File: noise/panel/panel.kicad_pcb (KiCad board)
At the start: 2 copper layers, 33 x 99.1 mm, 4 parts

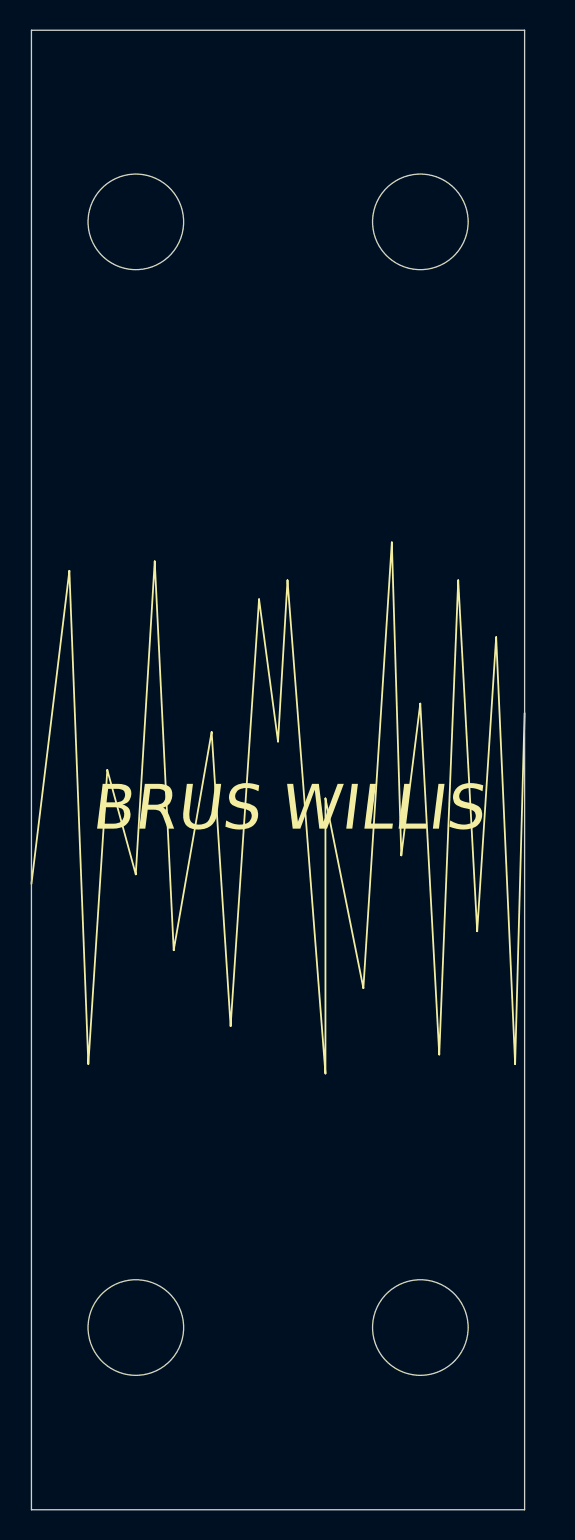
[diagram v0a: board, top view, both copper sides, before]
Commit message: Changes
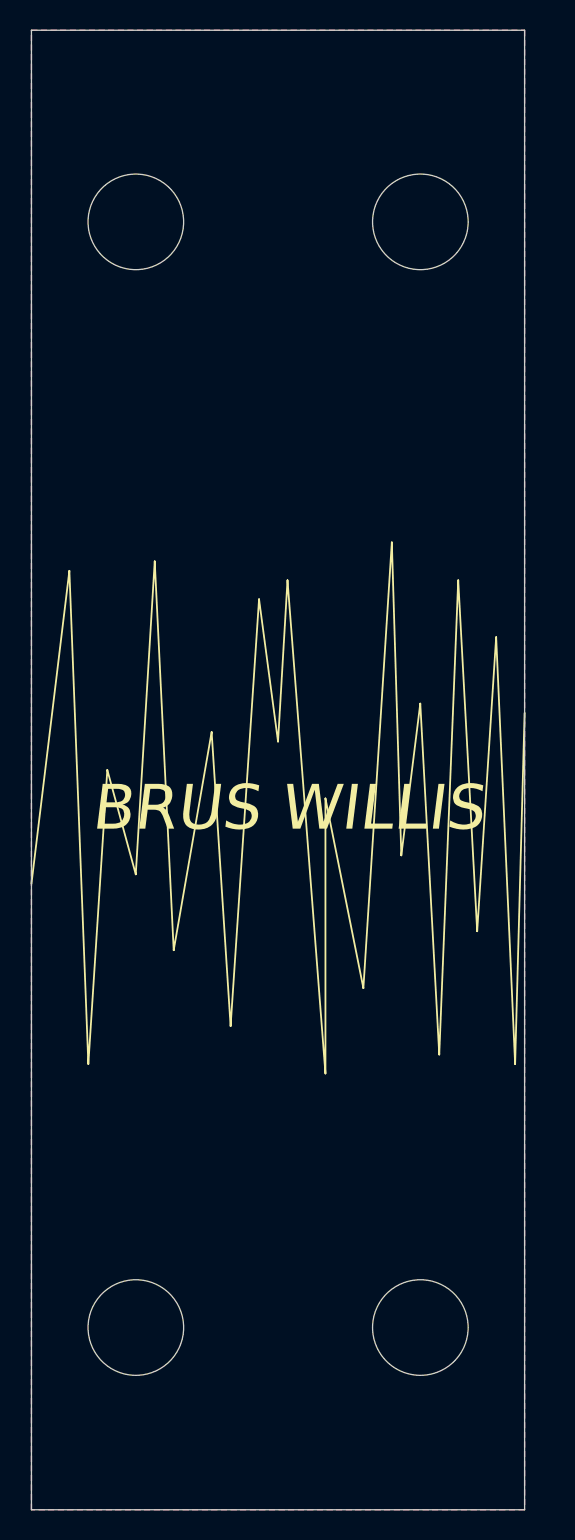
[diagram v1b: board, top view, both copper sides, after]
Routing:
- added copper zone on B.Cu, net (none)
- added copper zone on F.Cu, net (none)
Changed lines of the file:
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@@
   (general
     (thickness 1.6)
-    (drawings 29)
+    (drawings 28)
     (tracks 0)
     (zones 0)
@@
     (pcbplotparams
       (layerselection 0x010fc_ffffffff)
-      (usegerberextensions false)
-      (usegerberattributes true)
-      (usegerberadvancedattributes true)
-      (creategerberjobfile true)
+      (usegerberextensions true)
+      (usegerberattributes false)
+      (usegerberadvancedattributes false)
+      (creategerberjobfile false)
       (excludeedgelayer true)
       (linewidth 0.100000)
@@
       (plotinvisibletext false)
       (padsonsilk false)
-      (subtractmaskfromsilk false)
+      (subtractmaskfromsilk true)
       (outputformat 1)
       (mirror false)
-      (drillshape 1)
+      (drillshape 0)
       (scaleselection 1)
-      (outputdirectory ""))
+      (outputdirectory "plot"))
   )
   (net 0 "")
@@
       (effects (font (size 1 1) (thickness 0.15)))
     )
-    (fp_text user %R (at 0.3 0) (layer F.Fab) hide
-      (effects (font (size 1 1) (thickness 0.15)))
-    )
-    (fp_circle (center 0 0) (end 6.4 0) (layer Cmts.User) (width 0.15))
-    (fp_circle (center 0 0) (end 6.65 0) (layer F.CrtYd) (width 0.05))
+    (fp_circle (center 0 0) (end 6.4 0) (layer Cmts.User) (width 0.15))
+    (fp_circle (center 0 0) (end 6.65 0) (layer F.CrtYd) (width 0.05))
+    (fp_text user %R (at 0.3 0) (layer F.Fab) hide
+      (effects (font (size 1 1) (thickness 0.15)))
+    )
     (pad 1 np_thru_hole circle (at 0 0) (size 6.4 6.4) (drill 6.4) (layers *.Cu *.Mask))
   )
@@
       (effects (font (size 1 1) (thickness 0.15)))
     )
-    (fp_text user %R (at 0.3 0) (layer F.Fab) hide
-      (effects (font (size 1 1) (thickness 0.15)))
-    )
-    (fp_circle (center 0 0) (end 6.4 0) (layer Cmts.User) (width 0.15))
-    (fp_circle (center 0 0) (end 6.65 0) (layer F.CrtYd) (width 0.05))
+    (fp_circle (center 0 0) (end 6.4 0) (layer Cmts.User) (width 0.15))
+    (fp_circle (center 0 0) (end 6.65 0) (layer F.CrtYd) (width 0.05))
+    (fp_text user %R (at 0.3 0) (layer F.Fab) hide
+      (effects (font (size 1 1) (thickness 0.15)))
+    )
     (pad 1 np_thru_hole circle (at 0 0) (size 6.4 6.4) (drill 6.4) (layers *.Cu *.Mask))
   )
@@
   (gr_line (start 53.34 80.645) (end 54.61 113.665) (layer F.SilkS) (width 0.12))
   (gr_line (start 50.8 101.6) (end 53.34 80.645) (layer F.SilkS) (width 0.12))
-  (target plus (at 50.8 44.45) (size 5) (width 0.05) (layer Edge.Cuts))
   (gr_line (start 50.8 143.51) (end 50.8 44.45) (layer Edge.Cuts) (width 0.05))
   (gr_line (start 83.82 143.51) (end 50.8 143.51) (layer Edge.Cuts) (width 0.05))
   (gr_line (start 83.82 44.45) (end 83.82 143.51) (layer Edge.Cuts) (width 0.05))
   (gr_line (start 50.8 44.45) (end 83.82 44.45) (layer Edge.Cuts) (width 0.05))
+  (zone (net 0) (net_name "") (layer F.Cu) (hatch edge 0.508)
+    (connect_pads (clearance 0.508))
+    (min_thickness 0.254)
+    (fill yes (arc_segments 32) (thermal_gap 0.508) (thermal_bridge_width 0.508))
+    (polygon
+      (pts
+        (xy 83.82 143.51) (xy 50.8 143.51) (xy 50.8 44.45) (xy 83.82 44.45)
+      )
+    )
+  )
+  (zone (net 0) (net_name "") (layer B.Cu) (hatch edge 0.508)
+    (connect_pads (clearance 0.508))
+    (min_thickness 0.254)
+    (fill yes (arc_segments 32) (thermal_gap 0.508) (thermal_bridge_width 0.508))
+    (polygon
+      (pts
+        (xy 83.82 143.51) (xy 50.8 143.51) (xy 50.8 44.45) (xy 83.82 44.45)
+      )
+    )
+  )
 )
